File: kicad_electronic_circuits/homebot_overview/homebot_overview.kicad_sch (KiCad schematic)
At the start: 9 parts, among them J1 Raspberry_Pi_4, U1 TB6612FNG, U2 BNO055, U4 PCA9685BS

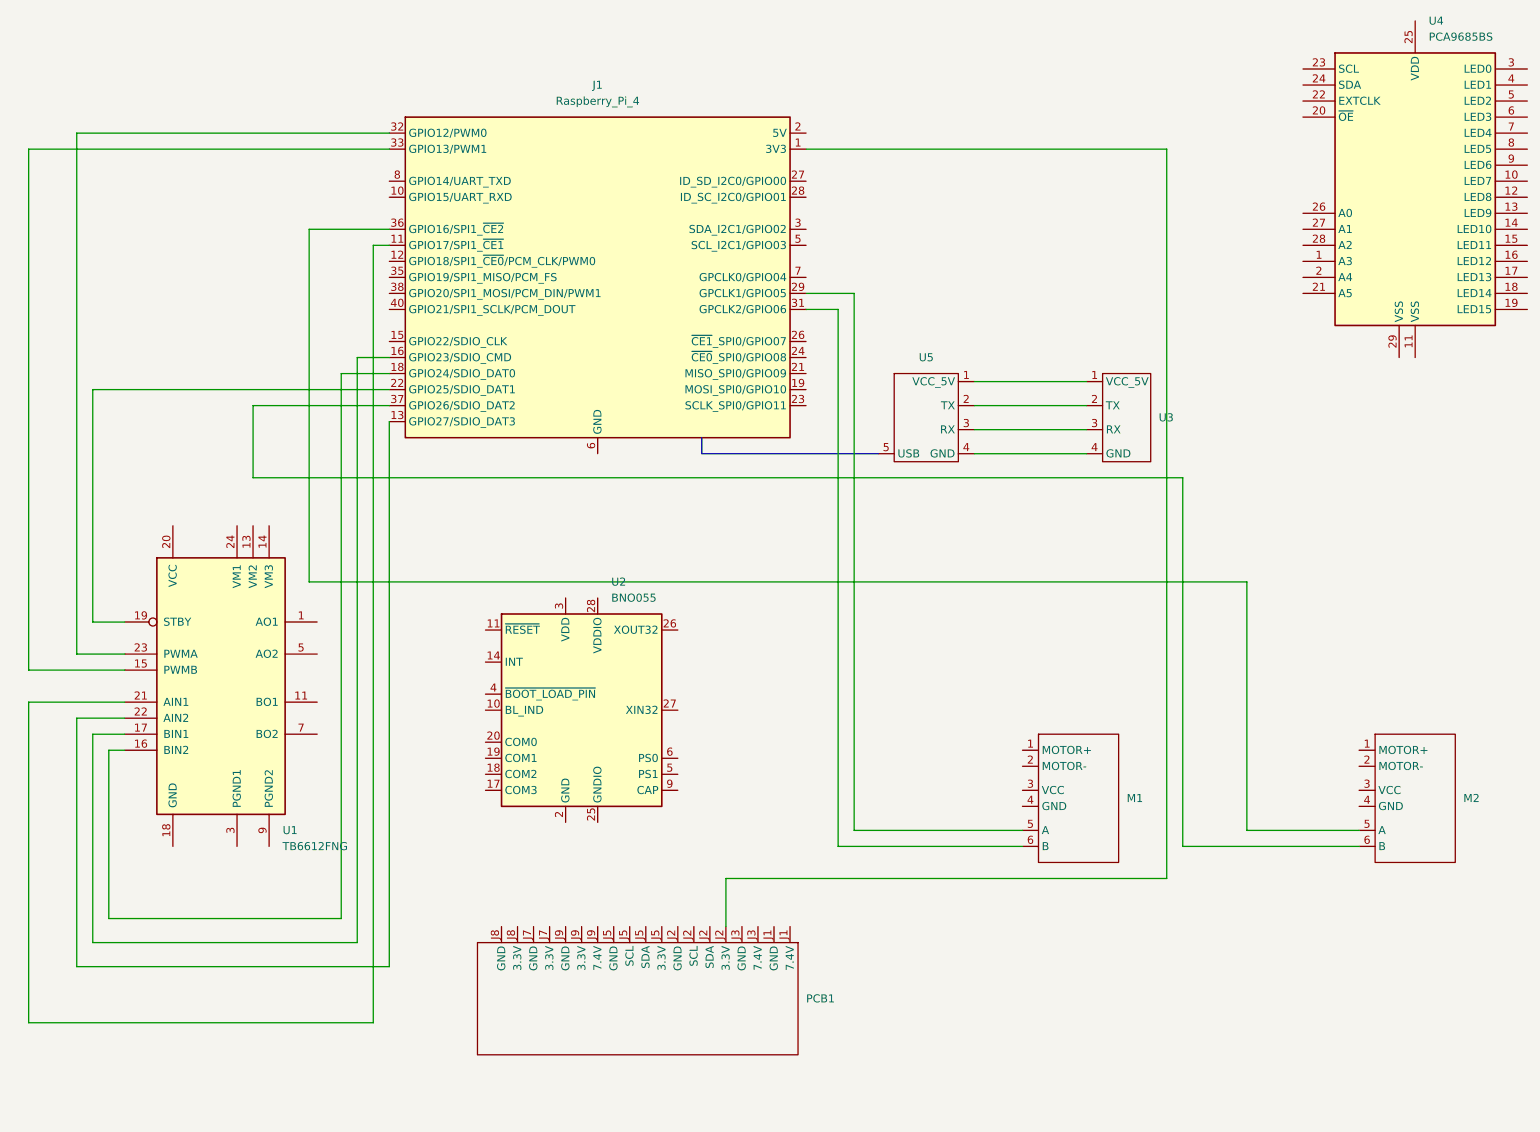
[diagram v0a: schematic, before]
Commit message: wrapped up electrical overview
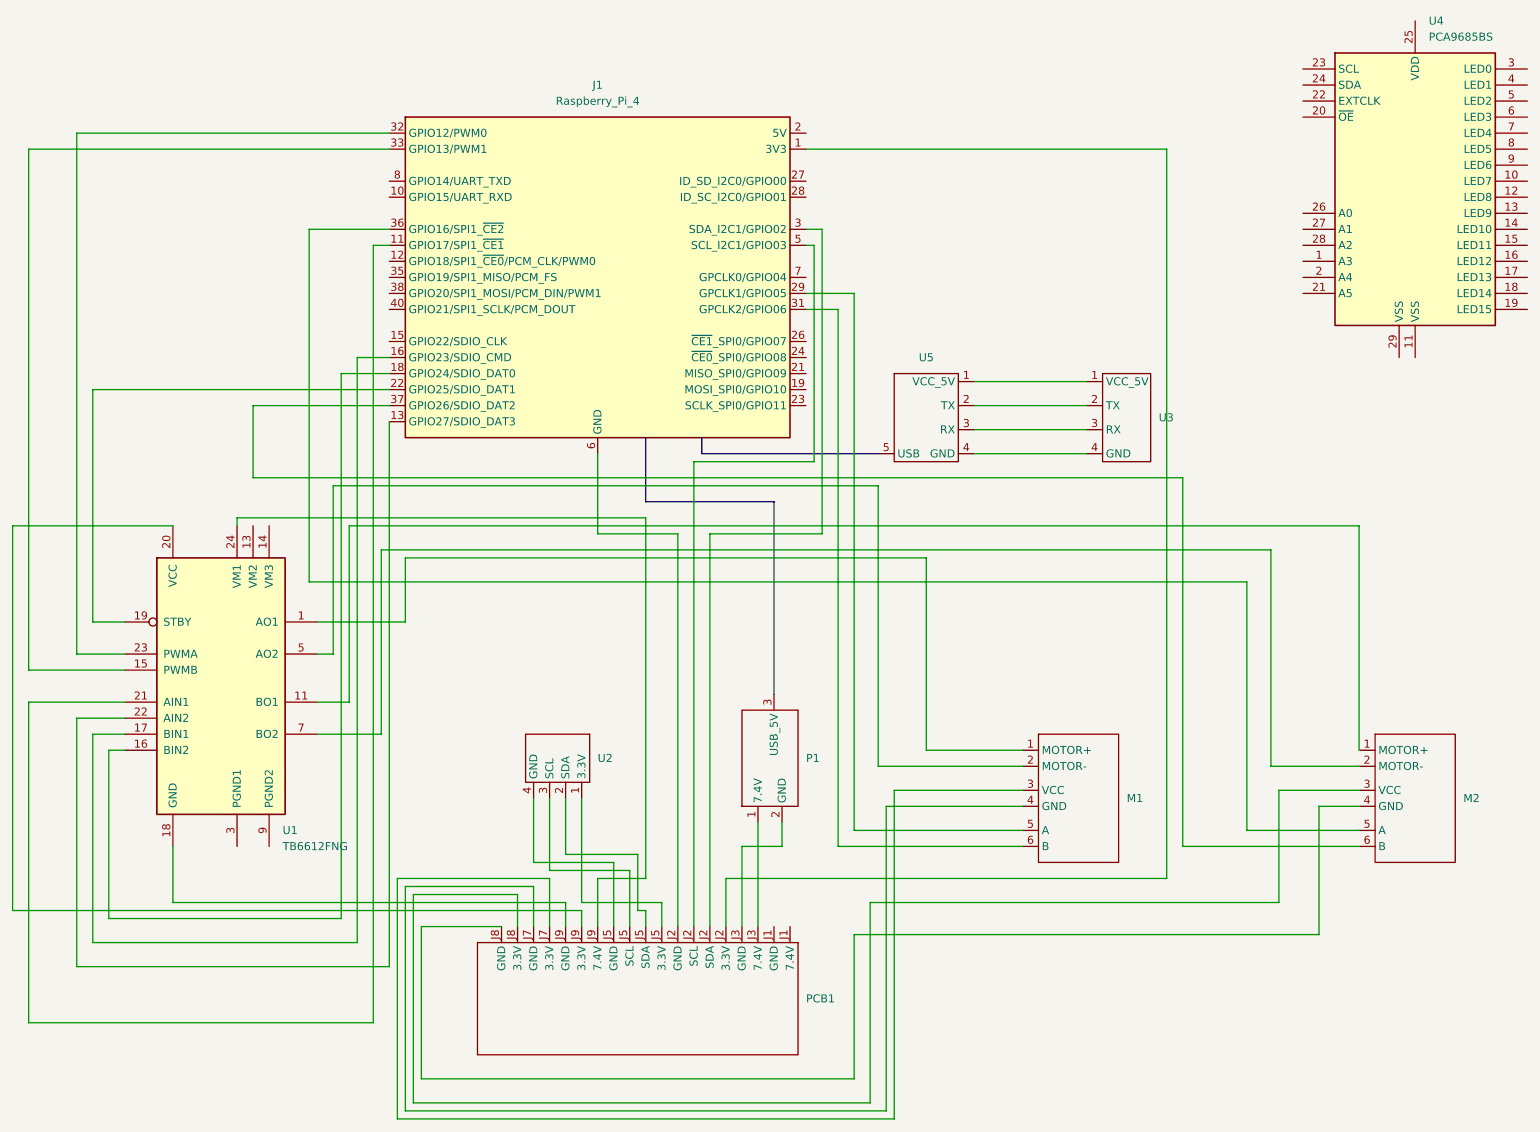
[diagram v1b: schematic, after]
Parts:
- removed U2: BNO055, Package_LGA:LGA-28_5.2x3.8mm_P0.5mm, symbol Sensor_Motion:BNO055
- added P1: (no value), symbol homebot_symbols:Buck_converter_7.4V_to_5V
- added U2: (no value), symbol homebot_symbols:BNO055_Module
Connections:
- net at U1.1 (AO1), U1.2 (AO1): now also M1.1 (MOTOR+)
- net at U1.11 (BO1), U1.12 (BO1): now also M2.1 (MOTOR+)
- net at U1.18 (GND): now also PCB1.J9 (GND)
- net at U1.20 (VCC): now also PCB1.J9 (GND)
- net at U1.24 (VM1): now also PCB1.J9 (GND)
- net at U1.5 (AO2), U1.6 (AO2): now also M1.2 (MOTOR-)
- net at U1.7 (BO2), U1.8 (BO2): now also M2.2 (MOTOR-)
- net at PCB1.J2 (GND): now also J1.5 (SCL_I2C1/GPIO03)
- net at PCB1.J3 (GND): now also P1.2 (GND)
- net at PCB1.J5 (GND): now also U2.4 (GND)
- net at PCB1.J7 (GND): now also M1.4 (GND)
- net at PCB1.J8 (GND): now also M2.4 (GND)
- net at J1.14 (GND), J1.20 (GND), J1.25 (GND)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: now also PCB1.J2 (GND)
- net at J1.3 (SDA_I2C1/GPIO02): now also PCB1.J2 (GND)
- net at M1.3 (VCC): now also PCB1.J7 (GND)
- net at M2.3 (VCC): now also PCB1.J8 (GND)
- new net: P1.1 (7.4V), PCB1.J3 (GND)
- new net: PCB1.J5 (GND), U2.1 (3.3V)
- new net: PCB1.J5 (GND), U2.2 (SDA)
- new net: PCB1.J5 (GND), U2.3 (SCL)
